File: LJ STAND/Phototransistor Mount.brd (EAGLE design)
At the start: 22 x 15 mm, 6 parts, among them IC1 A1301LH, IC2 A1301LH

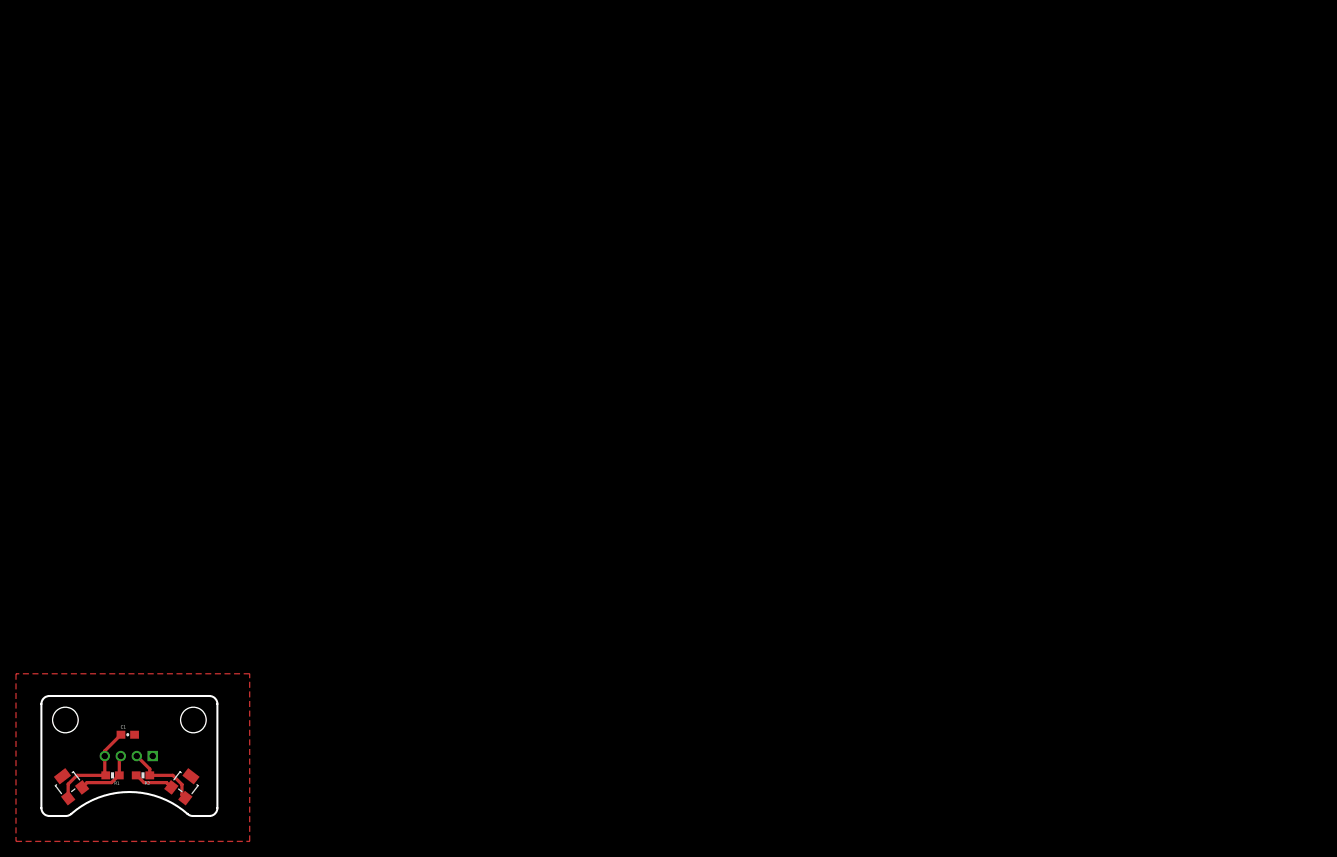
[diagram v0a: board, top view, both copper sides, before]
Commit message: Main edits, light gate pcbs
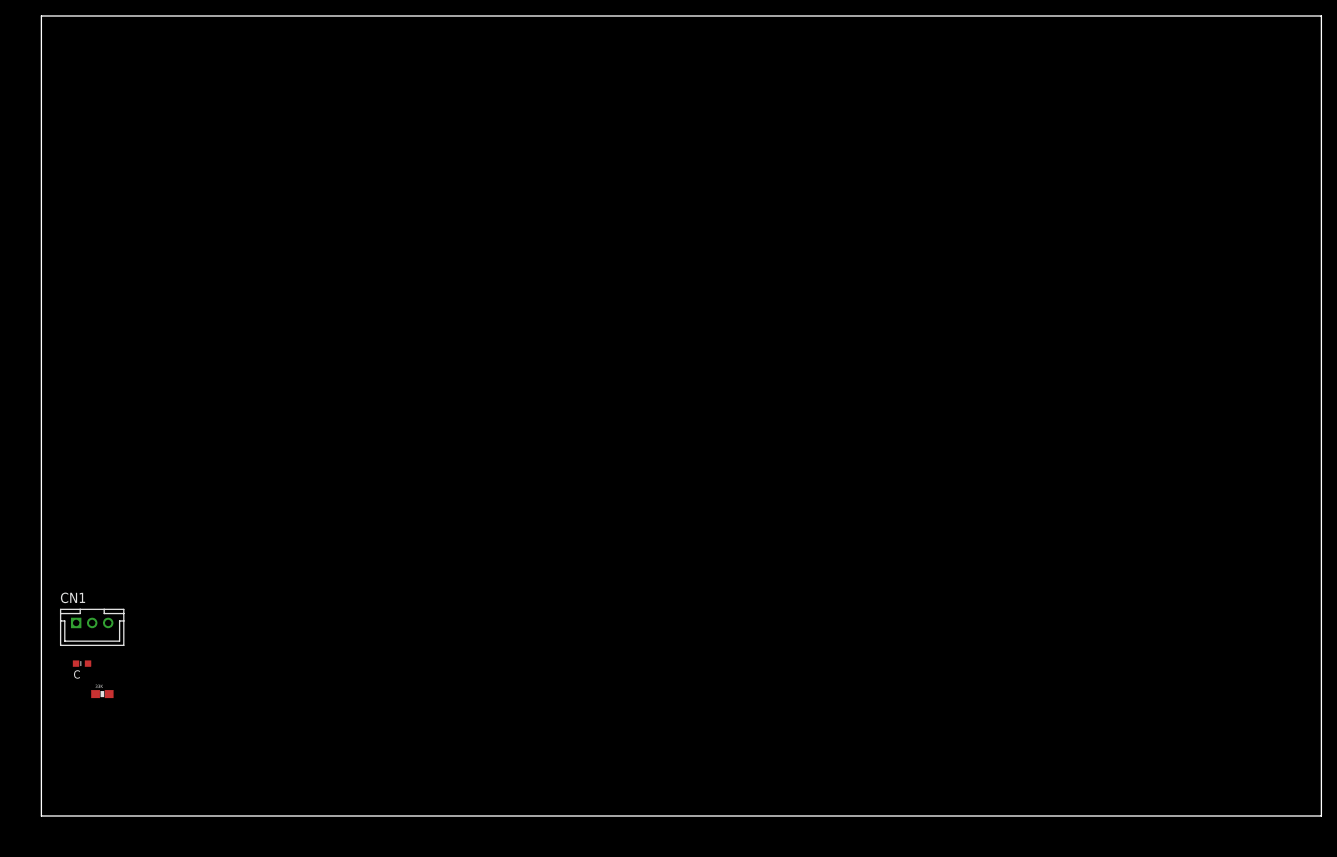
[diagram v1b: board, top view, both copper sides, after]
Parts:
- removed C1: 0.1uF, SparkFun-Capacitors:0603-CAP
- removed IC1, IC2: A1301LH, allegro:SOT23-W
- removed J1: (no value), jst-ph:B4B-PH-K-S
- removed R1, R2: 10K, SparkFun-Resistors:0603-RES
- added 33K: (no value), SparkFun-Passives:0603-RES
- added CN1: (no value), jst-ph:B3B-PH-K-S
- added U$1: ALS, phototransitor-ALS-PT19-315CL177TR8:SMD
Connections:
- removed net GND: C1.2, IC1.3, IC2.3, J1.1
- removed net OUTA: IC1.2, J1.3, R1.1
- removed net OUTB: IC2.2, J1.2, R2.1
- removed net VCC: C1.1, IC1.1, IC2.1, J1.4, R1.2, R2.2
- new net N$1: CN1.3, U$1.C
- new net N$2: 33K.1, CN1.1
- new net OUT: 33K.2, CN1.2, U$1.E
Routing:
- net VCC: track 18.0 -> 0.00 mm
- net OUTB: track 9.46 -> 0.00 mm
- net OUTA: track 7.76 -> 0.00 mm
- removed copper zone on layer 1, net GND
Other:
- board size 22 x 15 mm -> 160 x 100 mm
